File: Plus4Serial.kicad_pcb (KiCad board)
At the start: 2 copper layers, 54 x 47.5 mm, 11 parts, among them CN1 C64-User-Port-Female, CN2 DB9_MALE, U1 MC1489, U2 MC1488

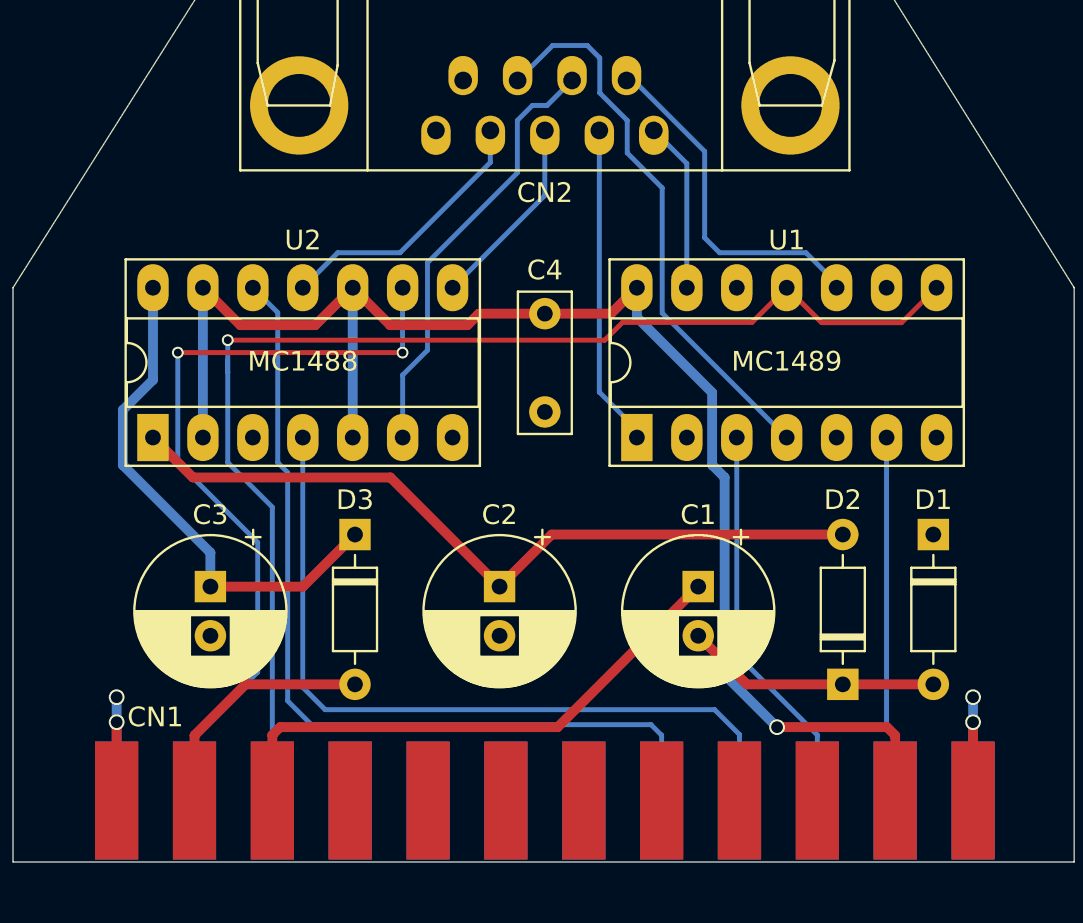
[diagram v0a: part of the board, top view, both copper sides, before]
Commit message: Fix some errors
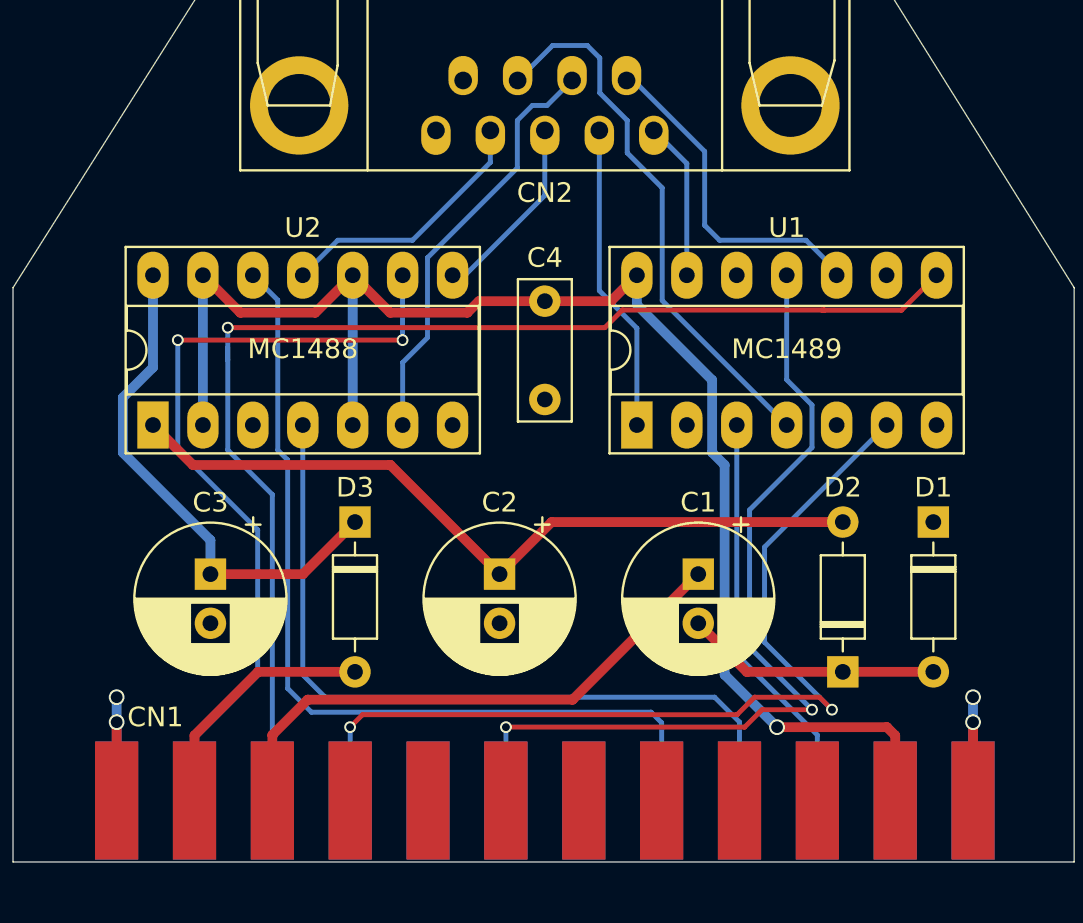
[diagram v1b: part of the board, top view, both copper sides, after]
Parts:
- CN1: value C64-User-Port-Female -> PLUS4_USERPORT
- moved C1 0.64 mm to (160.1, 102.7)
- moved C2 0.64 mm to (150.0, 102.7)
- moved C3 0.64 mm to (135.3, 102.7)
- moved C4 0.64 mm to (152.3, 88.8)
- moved D1 0.64 mm to (172.0, 100.1)
- moved D2 0.64 mm to (167.4, 107.7)
- moved D3 0.64 mm to (142.6, 100.1)
- moved U1 0.63 mm to (157.0, 95.1)
- moved U2 0.63 mm to (132.3, 95.1)
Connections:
- net /_dcd renamed /_~dcd
- CN1 pad 3: Net-(CN1-Pad3) -> (no net)
- CN1 pad 4: Net-(CN1-Pad4) -> (no net)
- CN1 pad 5: Net-(CN1-Pad5) -> (no net)
- CN1 pad 6: Net-(CN1-Pad6) -> (no net)
- CN1 pad 7: Net-(CN1-Pad7) -> (no net)
- CN1 pad 8: /rxc -> (no net)
- CN1 pad 9: Net-(CN1-Pad9) -> (no net)
- CN1 pad B: /~cts -> (no net)
- CN1 pad F: Net-(CN1-PadF) -> (no net)
- CN1 pad J: Net-(CN1-PadJ) -> (no net)
- CN1 pad K: Net-(CN1-PadK) -> /~cts
- CN2 pad 9: /_ri -> (no net)
- U1 pad 11: /~dsr -> /~dcd
- U1 pad 12: Net-(U1-Pad12) -> (no net)
- U1 pad 2: Net-(U1-Pad2) -> (no net)
- U1 pad 5: Net-(U1-Pad5) -> (no net)
- U1 pad 9: Net-(U1-Pad9) -> (no net)
- U2 pad 3: Net-(U2-Pad3) -> (no net)
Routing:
- net /~dcd: track 0.00 -> 45.0 mm, vias 0 -> 2
- net /~cts: track 18.6 -> 47.6 mm, vias 0 -> 2
- net /~dsr: track 63.6 -> 62.9 mm
- net +5V: track 75.3 -> 75.9 mm
- net /~dtr: track 44.8 -> 45.5 mm
- net /_~dsr: track 17.8 -> 17.1 mm
- net /txd: track 40.5 -> 41.2 mm
- net /_~rts: track 22.2 -> 21.5 mm
- net /~rts: track 39.3 -> 39.9 mm
- net /rxd: track 20.2 -> 20.8 mm
- net /_~cts: track 28.4 -> 27.8 mm
- net /_rxd: track 16.4 -> 15.8 mm
